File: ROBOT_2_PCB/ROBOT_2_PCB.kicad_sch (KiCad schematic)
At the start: 32 parts, among them J1 Bluetooth, U1 ULN2003

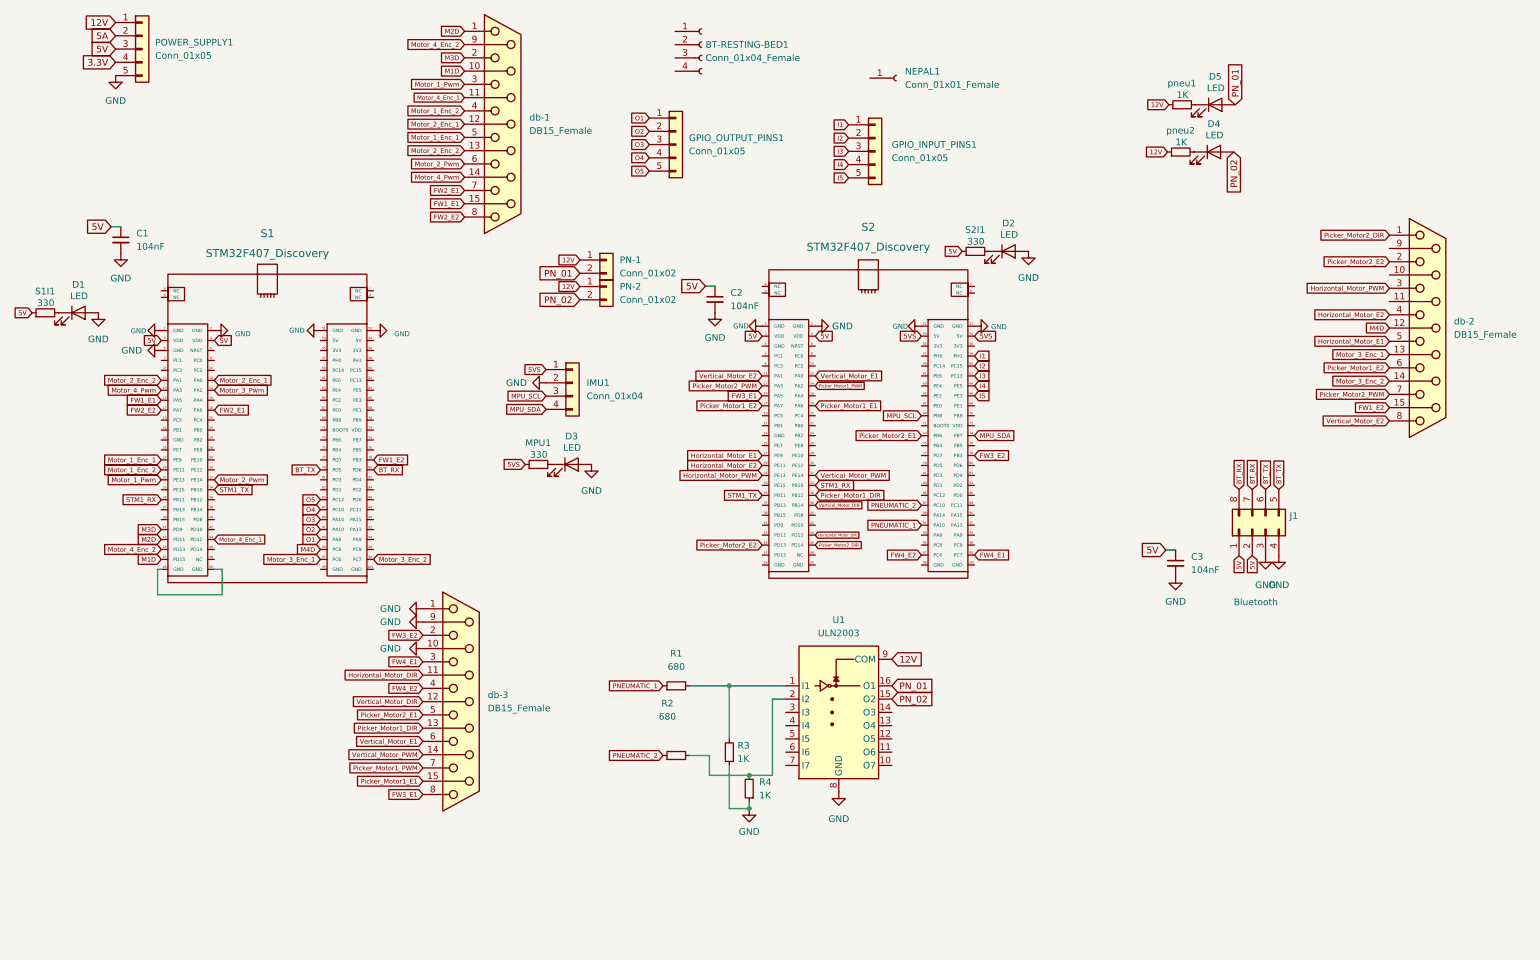
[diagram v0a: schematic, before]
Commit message: Push All
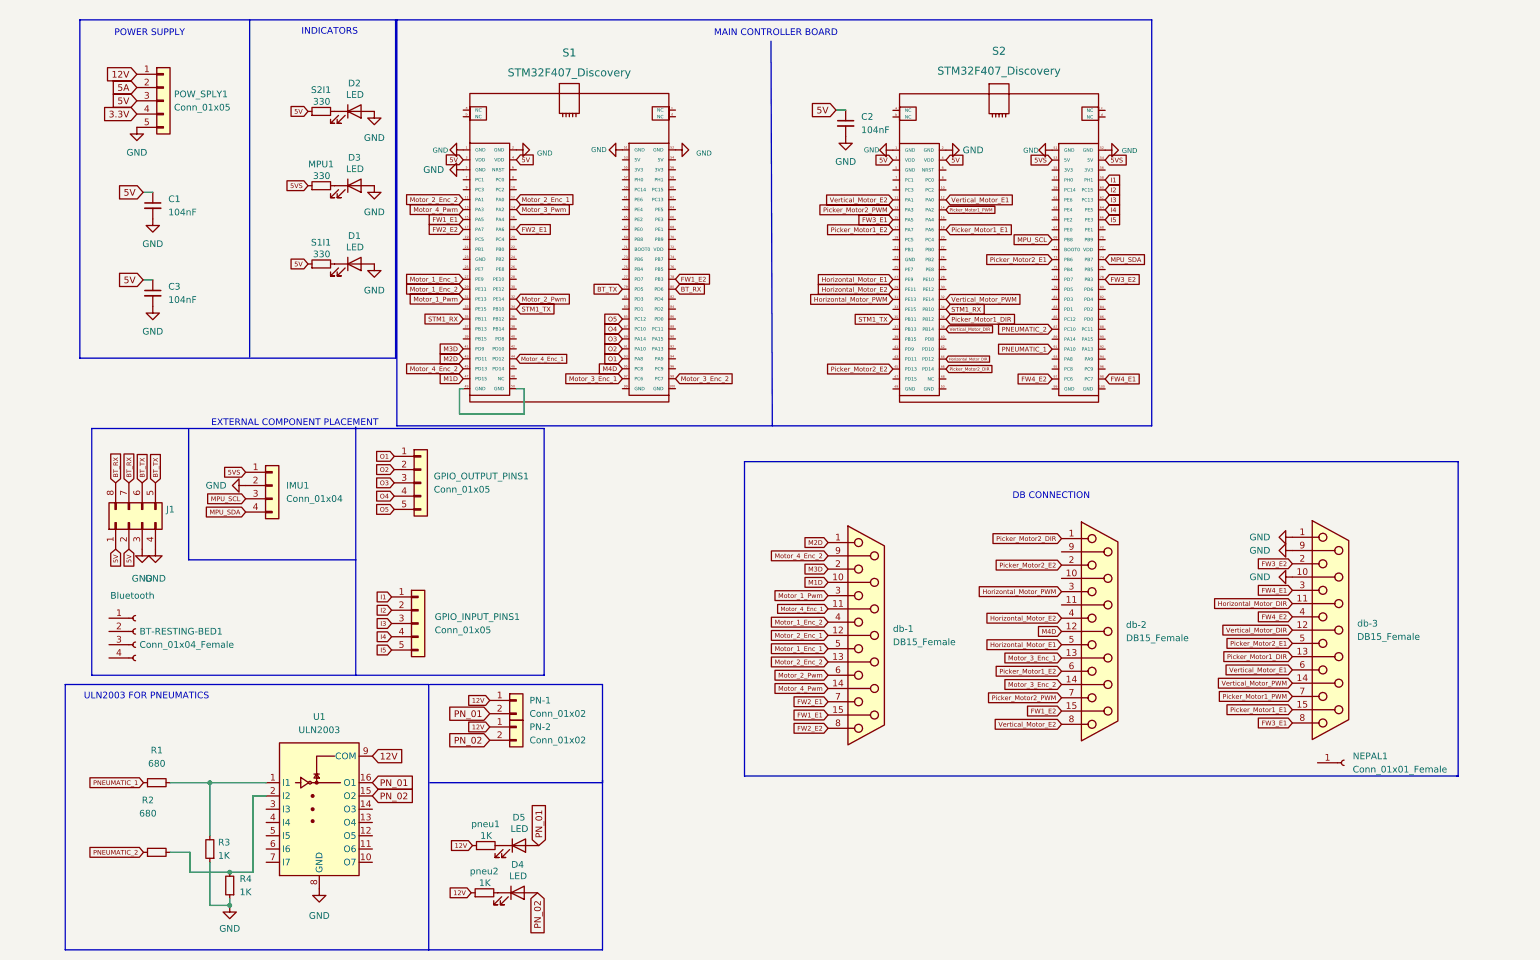
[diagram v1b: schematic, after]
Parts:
- renumbered POWER_SUPPLY1 to POW_SPLY1
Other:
- note added: "DB CONNECTION"
- note added: "EXTERNAL COMPONENT PLACEMENT"
- note added: "INDICATORS"
- note added: "MAIN CONTROLLER BOARD"
- note added: "POWER SUPPLY"
- note added: "ULN2003 FOR PNEUMATICS"
- moved on the sheet: BT-RESTING-BED1, C1, C2, C3, D1, D2, D3, D4, D5, GPIO_INPUT_PINS1, GPIO_OUTPUT_PINS1, IMU1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
